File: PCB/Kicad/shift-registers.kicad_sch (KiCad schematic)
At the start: 7 parts

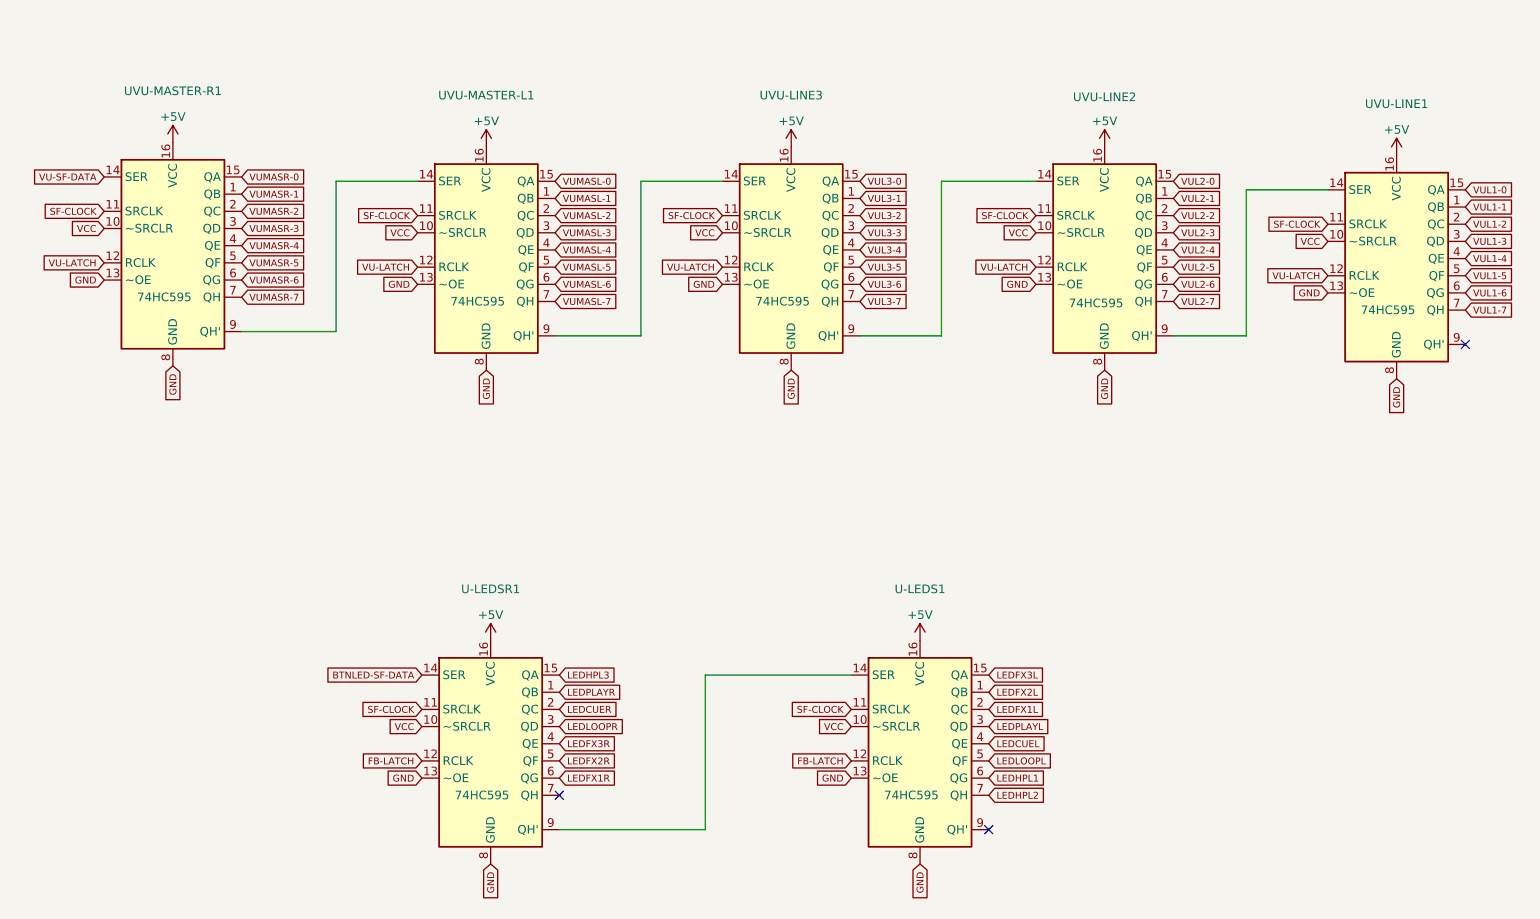
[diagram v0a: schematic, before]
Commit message: SCHEMATIC FINISHED
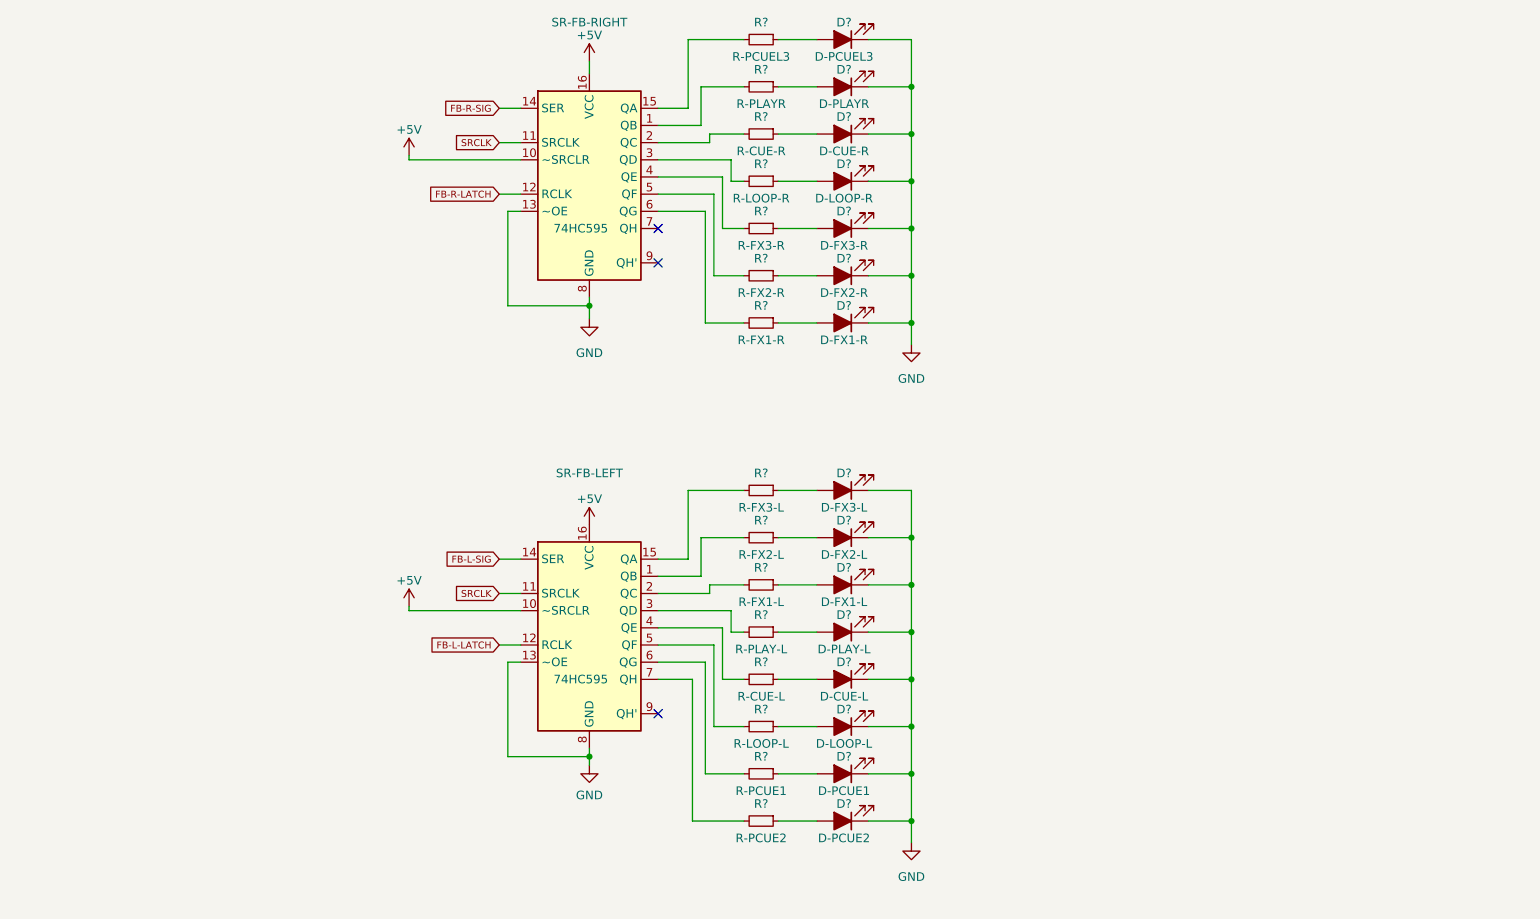
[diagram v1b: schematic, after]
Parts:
- removed UVU-LINE1, UVU-LINE2, UVU-LINE3, UVU-MASTER-L1, UVU-MASTER-R1: 74HC595, Library:SO-16_3.9x9.9mm_P1.27mm, symbol 74xx:74HC595
- added D?: D-PLAY-L, Library:LED_GREEN, symbol Device:LED_Filled
- added D?: D-FX2-R, Library:LED_GREEN, symbol Device:LED_Filled
- added D?: D-FX2-L, Library:LED_GREEN, symbol Device:LED_Filled
- added D?: D-PCUEL3, Library:LED_GREEN, symbol Device:LED_Filled
- added D?: D-FX1-R, Library:LED_GREEN, symbol Device:LED_Filled
- added D?: D-FX3-R, Library:LED_GREEN, symbol Device:LED_Filled
- added D?: D-LOOP-R, Library:LED_GREEN, symbol Device:LED_Filled
- added D?: D-PCUE1, Library:LED_GREEN, symbol Device:LED_Filled
- added D?: D-PCUE2, Library:LED_GREEN, symbol Device:LED_Filled
- added D?: D-CUE-L, Library:LED_GREEN, symbol Device:LED_Filled
- added D?: D-CUE-R, Library:LED_GREEN, symbol Device:LED_Filled
- added D?: D-FX1-L, Library:LED_GREEN, symbol Device:LED_Filled
- added D?: D-PLAYR, Library:LED_GREEN, symbol Device:LED_Filled
- added D?: D-LOOP-L, Library:LED_GREEN, symbol Device:LED_Filled
- added D?: D-FX3-L, Library:LED_GREEN, symbol Device:LED_Filled
- added R?: R-PCUEL3, Library:R_1206_3216Metric_Pad1.30x1.75mm_HandSolder, symbol Device:R_Small
- added R?: R-FX1-R, Library:R_1206_3216Metric_Pad1.30x1.75mm_HandSolder, symbol Device:R_Small
- added R?: R-FX3-L, Library:R_1206_3216Metric_Pad1.30x1.75mm_HandSolder, symbol Device:R_Small
- added R?: R-LOOP-L, Library:R_1206_3216Metric_Pad1.30x1.75mm_HandSolder, symbol Device:R_Small
- added R?: R-LOOP-R, Library:R_1206_3216Metric_Pad1.30x1.75mm_HandSolder, symbol Device:R_Small
- added R?: R-CUE-R, Library:R_1206_3216Metric_Pad1.30x1.75mm_HandSolder, symbol Device:R_Small
- added R?: R-PCUE2, Library:R_1206_3216Metric_Pad1.30x1.75mm_HandSolder, symbol Device:R_Small
- added R?: R-CUE-L, Library:R_1206_3216Metric_Pad1.30x1.75mm_HandSolder, symbol Device:R_Small
- added R?: R-FX1-L, Library:R_1206_3216Metric_Pad1.30x1.75mm_HandSolder, symbol Device:R_Small
- added R?: R-PCUE1, Library:R_1206_3216Metric_Pad1.30x1.75mm_HandSolder, symbol Device:R_Small
- added R?: R-FX2-R, Library:R_1206_3216Metric_Pad1.30x1.75mm_HandSolder, symbol Device:R_Small
- added R?: R-PLAYR, Library:R_1206_3216Metric_Pad1.30x1.75mm_HandSolder, symbol Device:R_Small
- added R?: R-FX2-L, Library:R_1206_3216Metric_Pad1.30x1.75mm_HandSolder, symbol Device:R_Small
- added R?: R-PLAY-L, Library:R_1206_3216Metric_Pad1.30x1.75mm_HandSolder, symbol Device:R_Small
- added R?: R-FX3-R, Library:R_1206_3216Metric_Pad1.30x1.75mm_HandSolder, symbol Device:R_Small
- renumbered U-LEDS1 to SR-FB-LEFT, U-LEDSR1 to SR-FB-RIGHT
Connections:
- net VCC is gone; now on net +5V: SR-FB-LEFT.10 (~SRCLR), SR-FB-RIGHT.10 (~SRCLR)
- net GND: now also D?.1 (K), D?.1 (K), D?.1 (K), D?.1 (K), D?.1 (K), D?.1 (K), D?.1 (K), D?.1 (K), D?.1 (K), D?.1 (K), D?.1 (K), D?.1 (K), D?.1 (K), D?.1 (K), D?.1 (K)
- net at SR-FB-RIGHT.9 (QH'): no longer SR-FB-LEFT.14 (SER)
- net BTNLED-SF-DATA renamed FB-R-SIG
- net FB-LATCH renamed FB-L-LATCH
- net FB-L-LATCH: no longer SR-FB-RIGHT.12 (RCLK)
- net LEDCUEL: no longer names the net of SR-FB-LEFT.4 (QE)
- net LEDCUEL: now also R?.2
- net LEDCUER: no longer names the net of SR-FB-RIGHT.2 (QC)
- net LEDCUER: now also R?.2
- net LEDFX1L: no longer names the net of SR-FB-LEFT.2 (QC)
- net LEDFX1L: now also R?.2
- net LEDFX1R: no longer names the net of SR-FB-RIGHT.6 (QG)
- net LEDFX1R: now also R?.2
- net LEDFX2L: no longer names the net of SR-FB-LEFT.1 (QB)
- net LEDFX2L: now also R?.2
- net LEDFX2R: no longer names the net of SR-FB-RIGHT.5 (QF)
- net LEDFX2R: now also R?.2
- net LEDFX3L: no longer names the net of SR-FB-LEFT.15 (QA)
- net LEDFX3L: now also R?.2
- net LEDFX3R: no longer names the net of SR-FB-RIGHT.4 (QE)
- net LEDFX3R: now also R?.2
- net LEDHPL1: no longer names the net of SR-FB-LEFT.6 (QG)
- net LEDHPL1: now also R?.2
- net LEDHPL2: no longer names the net of SR-FB-LEFT.7 (QH)
- net LEDHPL2: now also R?.2
- net LEDHPL3: no longer names the net of SR-FB-RIGHT.15 (QA)
- net LEDHPL3: now also R?.2
- net LEDLOOPL: no longer names the net of SR-FB-LEFT.5 (QF)
- net LEDLOOPL: now also R?.2
- net LEDLOOPR: no longer names the net of SR-FB-RIGHT.3 (QD)
- net LEDLOOPR: now also R?.2
- net LEDPLAYL: no longer names the net of SR-FB-LEFT.3 (QD)
- net LEDPLAYL: now also R?.2
- net LEDPLAYR: no longer names the net of SR-FB-RIGHT.1 (QB)
- net LEDPLAYR: now also R?.2
- net SF-CLOCK renamed SRCLK
- new net: D?.2 (A), R?.1 (x15)
- new net FB-L-SIG: SR-FB-LEFT.14 (SER)
- new net FB-R-LATCH: SR-FB-RIGHT.12 (RCLK)
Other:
- moved on the sheet: SR-FB-LEFT, SR-FB-RIGHT
